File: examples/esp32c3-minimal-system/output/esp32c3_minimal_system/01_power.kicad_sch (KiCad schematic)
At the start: 8 parts, among them J1 USB-C16PIN, U2 AMS1117-3.3

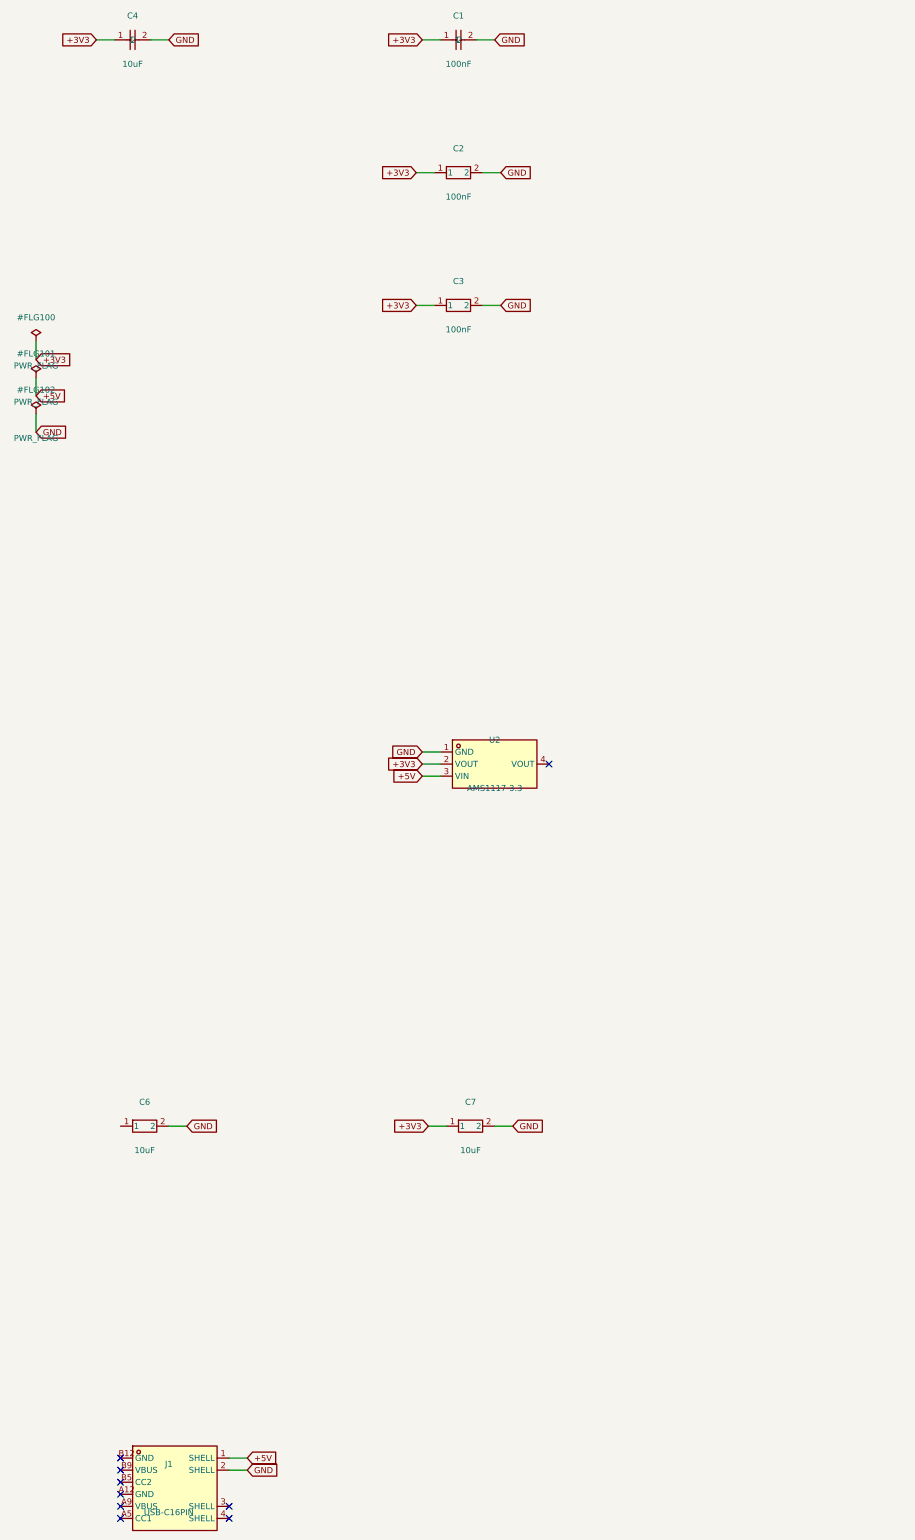
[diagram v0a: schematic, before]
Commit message: docs: refresh verified examples / 文档：刷新已验证示例
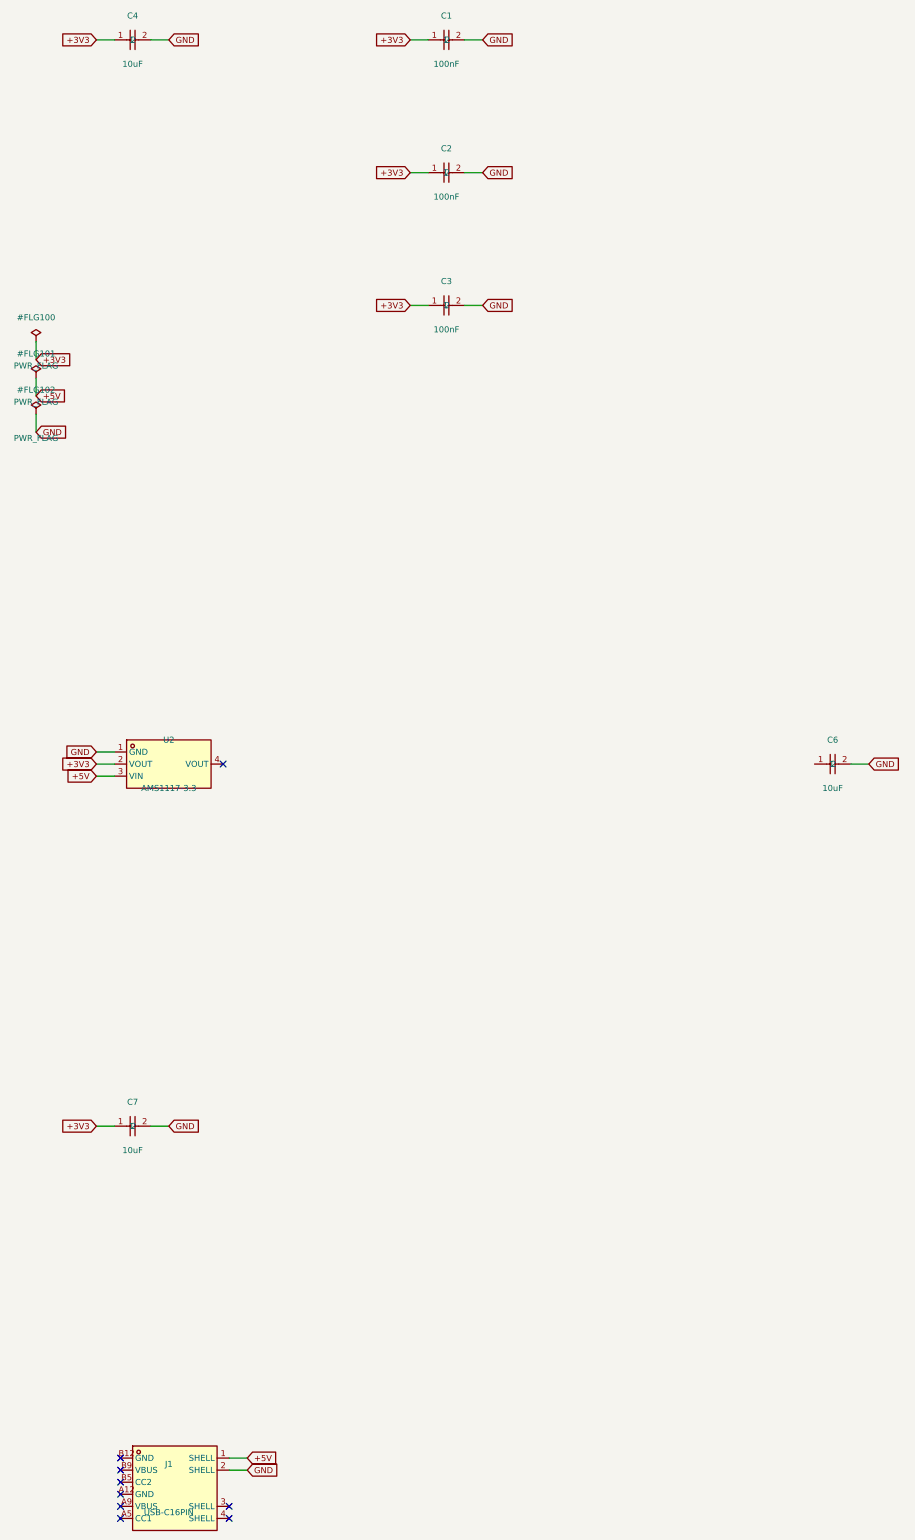
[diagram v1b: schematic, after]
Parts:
- removed C2, C3: 100nF, JLC-MCP:C0603, symbol JLC-MCP:C1590
- removed C6, C7: 10uF, JLC-MCP:C0805, symbol JLC-MCP:C1713
- added C2, C3: 100nF, JLC-MCP:C0603, symbol JLC-MCP:CL10B104KA8NNNC
- added C6, C7: 10uF, JLC-MCP:C0805, symbol JLC-MCP:CL21A106KOQNNNE
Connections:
- net +3V3: now also C2.1, C3.1, C7.1
- net GND: now also C2.2, C3.2, C6.2, C7.2
